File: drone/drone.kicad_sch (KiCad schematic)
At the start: 3 parts, among them U2 ESP32-DEVKIT-V1

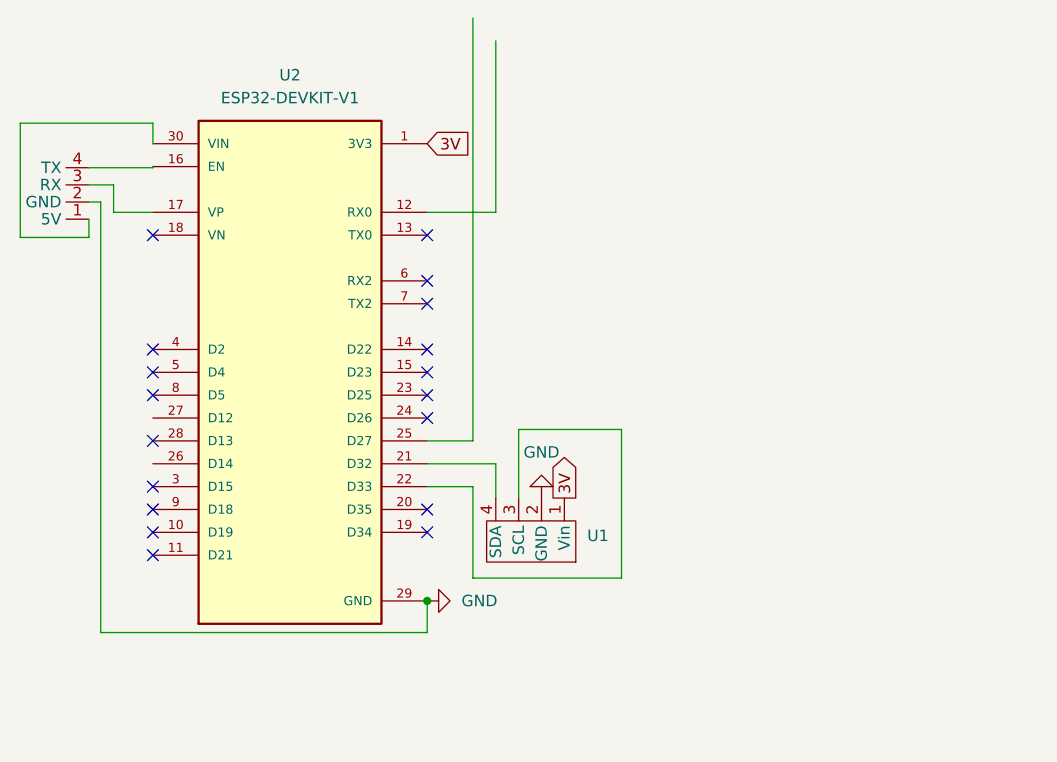
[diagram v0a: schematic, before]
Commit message: Fixed PCB
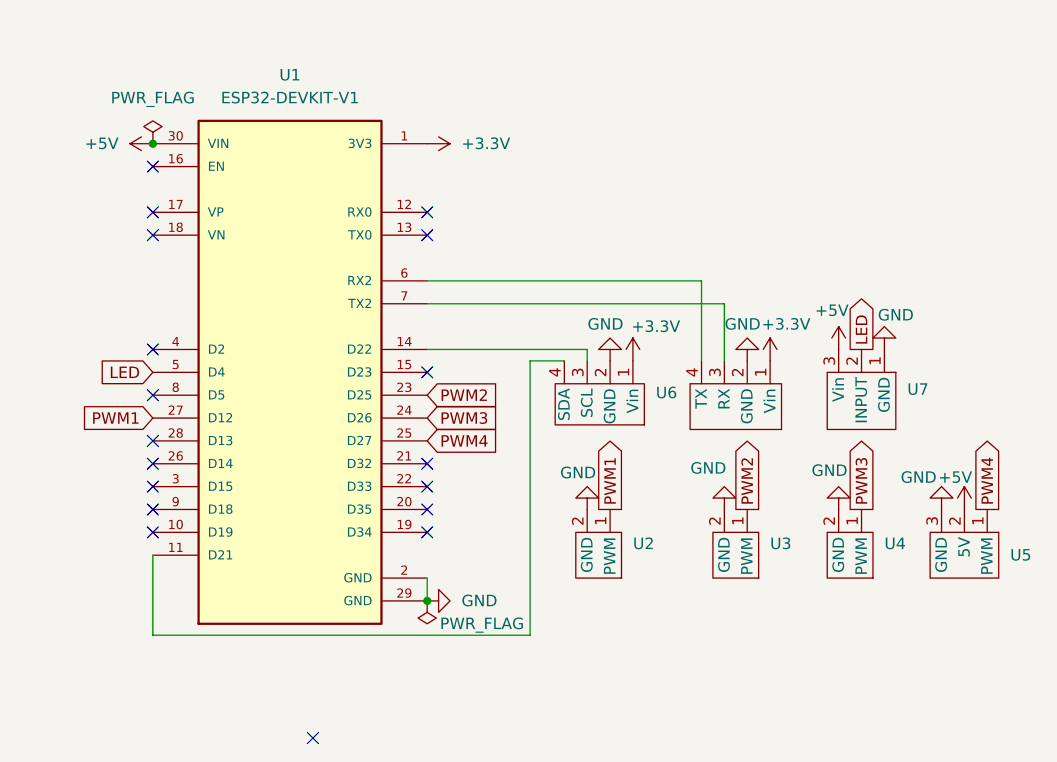
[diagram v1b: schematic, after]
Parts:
- removed L1: ~, Connector_PinHeader_2.54mm:PinHeader_1x04_P2.54mm_Vertical, symbol drone:lidar
- removed U1: ~, Connector_PinSocket_2.54mm:PinSocket_1x10_P2.54mm_Vertical, symbol drone:IMU
- removed U2: ESP32-DEVKIT-V1, esp32:MODULE_ESP32_DEVKIT_V1, symbol esp32:ESP32-DEVKIT-V1
- added L1: ~, Connector_PinSocket_2.54mm:PinSocket_1x04_P2.54mm_Vertical, symbol drone:LIDAR
- added U1: ESP32-DEVKIT-V1, ESP32:MODULE_ESP32_DEVKIT_V1, symbol ESP32:ESP32-DEVKIT-V1
- added U2, U3, U4: ~, Connector_PinSocket_2.54mm:PinSocket_1x02_P2.54mm_Vertical, symbol drone:ESC_Without5V
- added U5: ~, Connector_PinSocket_2.54mm:PinSocket_1x03_P2.54mm_Vertical, symbol drone:ESC
- added U6: ~, Connector_PinSocket_2.54mm:PinSocket_1x04_P2.54mm_Vertical, symbol drone:IMU
- added U7: ~, Connector_PinSocket_2.54mm:PinSocket_1x03_P2.54mm_Vertical, symbol drone:LED
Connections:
- net GND: now also L1.2 (GND), U1.2 (GND), U1.29 (GND), U2.2 (GND), U3.2 (GND), U4.2 (GND), U5.3 (GND), U6.2 (GND), U7.1 (GND)
- new net: L1.3 (RX), U1.7 (TX2)
- new net: L1.4 (TX), U1.6 (RX2)
- new net: U1.11 (D21), U6.4 (SDA)
- new net: U1.14 (D22), U6.3 (SCL)
- new net +3.3V: L1.1 (Vin), U1.1 (3V3), U6.1 (Vin)
- new net +5V: U1.30 (VIN), U5.2 (5V), U7.3 (Vin)
- new net LED: U1.5 (D4), U7.2 (INPUT)
- new net PWM1: U1.27 (D12), U2.1 (PWM)
- new net PWM2: U1.23 (D25), U3.1 (PWM)
- new net PWM3: U1.24 (D26), U4.1 (PWM)
- new net PWM4: U1.25 (D27), U5.1 (PWM)
